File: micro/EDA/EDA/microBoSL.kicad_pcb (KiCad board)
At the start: 4 copper layers, 40 x 13 mm, 37 parts, among them J1 Conn_01x04, J2 Conn_02x03_Odd_Even, J3 Conn_01x04, J4 Conn_01x04, J5 Conn_01x02, J6 Conn_01x10, J7 Conn_01x02, J8 USB_B_Micro, Q1 DMG2302UK, SW1 PTS636 SM43J SMTR LFS, U1 MAX40200ANS, U2 MAX40200ANS, U3 MCP1700-3302E_SOT23, U4 ATmega328-MMH, U5 MCP7940N-xSN, U6 74HC126PW-Q100, U7 FT232RQ, Y1 8MHz, Y2 32.768 kHz

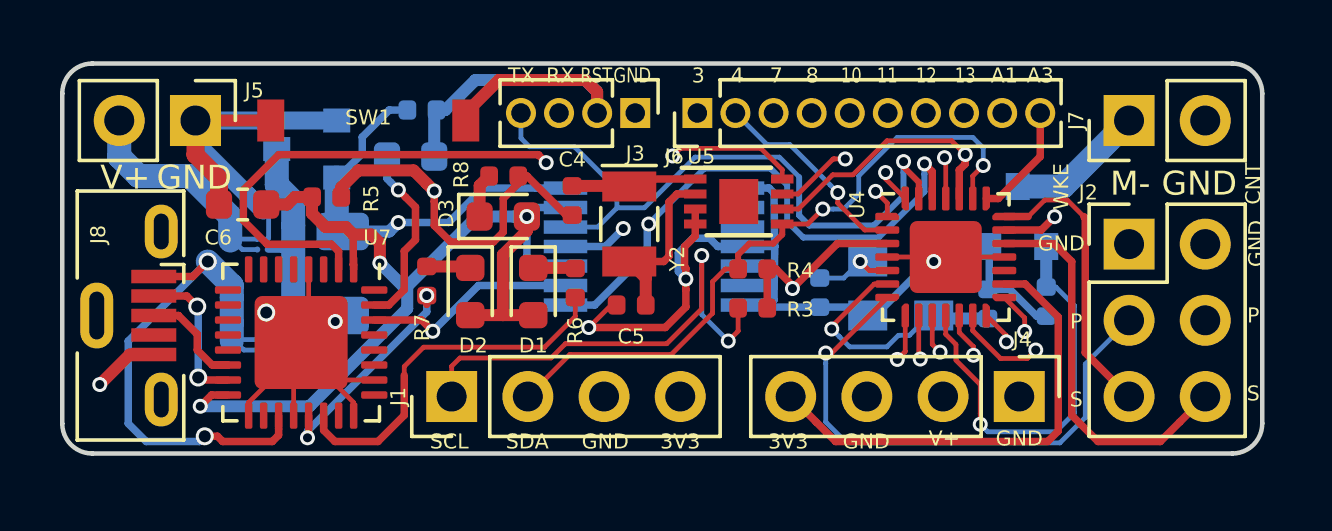
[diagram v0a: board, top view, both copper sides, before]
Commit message: microbosl layout finished TODO: optimise/silkscreen
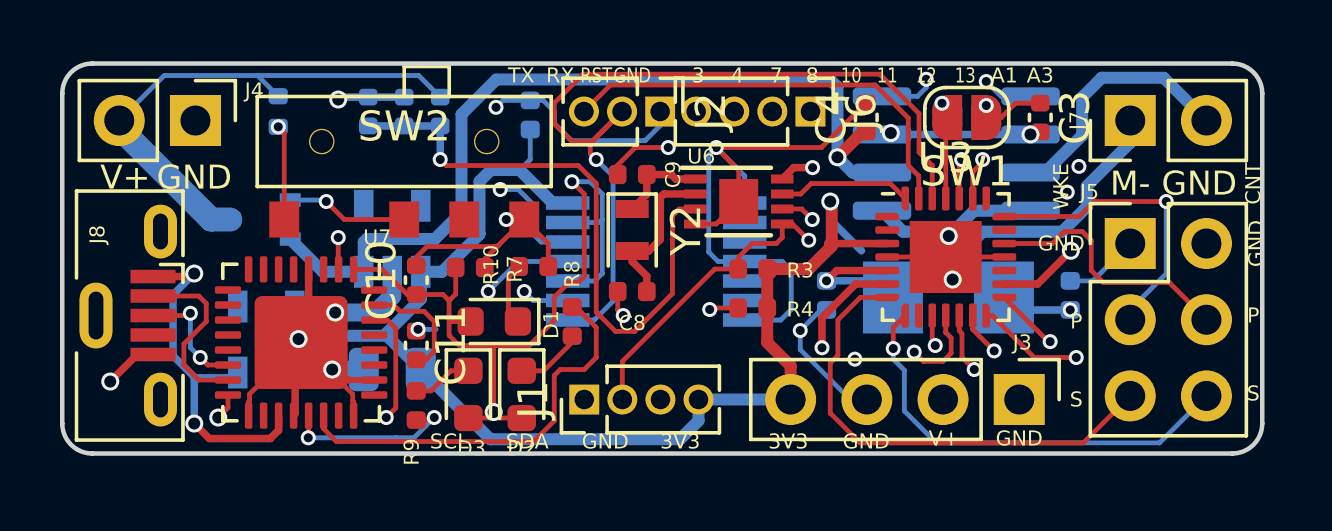
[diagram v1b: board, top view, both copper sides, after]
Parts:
- removed the C6 at (106.0, 106.7)
- removed the D3 at (114.7, 107.1)
- removed the J3 at (119.1, 103.7)
- removed the R2 at (132.8, 109.9)
- added C10: 100 nF, Capacitor_SMD:C_0402_1005Metric, F.Cu at (111.8, 109.2)
- added C11: 100 nF, Capacitor_SMD:C_0402_1005Metric, F.Cu at (111.8, 111.4)
- added C3: 100 nF, Capacitor_SMD:C_0402_1005Metric, F.Cu at (132.6, 103.8)
- added C4: 100 nF, Capacitor_SMD:C_0402_1005Metric, F.Cu at (126.8, 103.8)
- added D2: LED, LED_SMD:LED_0603_1608Metric, F.Cu at (115.3, 113.0)
- added J2: Conn_01x03, Connector_PinHeader_1.27mm:PinHeader_1x03_P1.27mm_Vertical, F.Cu at (119.9, 103.6)
- added R1: 10 kΩ, Resistor_SMD:R_0402_1005Metric, B.Cu at (107.2, 103.6)
- added R6: 4.7 MΩ, Capacitor_SMD:C_0402_1005Metric, B.Cu at (110.2, 103.6)
- added R9: 3.3 kΩ, Resistor_SMD:R_0402_1005Metric, F.Cu at (111.8, 113.4)
- added SW2: AYZ0103AGRLC, SIMFootprints:AYZ0103AGRLC, F.Cu at (111.4, 104.6)
- C1: value 1 μF -> 2.2 μF; footprint Capacitor_SMD:C_1206_3216Metric -> Capacitor_SMD:C_0805_2012Metric
- C5: renamed from C3; value 22 pF -> 15 pF
- C6: renamed from C2; value 22 pF -> 15 pF
- C7: footprint Capacitor_SMD:C_0603_1608Metric -> Capacitor_SMD:C_0402_1005Metric
- C8: renamed from C5; value 12 pF -> 15 pF
- C9: renamed from C4; value 12 pF -> 15 pF
- J1: footprint Connector_PinHeader_2.54mm:PinHeader_1x04_P2.54mm_Vertical -> Connector_PinHeader_1.27mm:PinHeader_1x04_P1.27mm_Vertical
- J4: renamed from J5; value Conn_01x02 -> BATTERY CONN
- J6: value Conn_01x10 -> Conn_01x04; footprint Connector_PinHeader_1.27mm:PinHeader_1x10_P1.27mm_Vertical -> Connector_PinHeader_1.27mm:PinHeader_1x04_P1.27mm_Vertical
- J7: value Conn_01x02 -> MOTOR_OUT
- Q1: value DMG2302UK -> DMP2165UW; footprint Package_TO_SOT_SMD:SOT-23 -> Package_TO_SOT_SMD:SOT-323_SC-70
- R5: value 10 kΩ -> 4.7 MΩ; footprint Resistor_SMD:R_0402_1005Metric -> Capacitor_SMD:C_0402_1005Metric; moved to B.Cu
- R7: value 3.3 kΩ -> 10 kΩ
- SW1: value PTS636 SM43J SMTR LFS -> RST_JMPR; footprint SIMFootprints:PTS636 SM43J SMTR LFS -> Jumper:SolderJumper-2_P1.3mm_Open_RoundedPad1.0x1.5mm
- U1, U2: value MAX40200ANS -> TPS709A33DBVT; footprint Package_BGA:WLP-4_0.73x0.73mm_Layout2x2_P0.35mm_Ball0.22mm_Pad0.2mm_NSMD -> Package_TO_SOT_SMD:SOT-23-5
- U3: value MCP1700-3302E_SOT23 -> ATmega328P-MMH; footprint Package_TO_SOT_SMD:SOT-23 -> Package_DFN_QFN:QFN-28-1EP_4x4mm_P0.45mm_EP2.4x2.4mm; moved to F.Cu
- U4: value ATmega328-MMH -> ZXBM5210-S; footprint Package_DFN_QFN:QFN-28-1EP_4x4mm_P0.45mm_EP2.4x2.4mm -> Package_SO:SOIC-8_3.9x4.9mm_P1.27mm; moved to B.Cu
- Y1: footprint Crystal:Crystal_SMD_EuroQuartz_MT-4Pin_3.2x2.5mm -> Crystal:Crystal_SMD_5032-2Pin_5.0x3.2mm
- Y2: footprint Crystal:Crystal_SMD_EuroQuartz_EQ161-2Pin_3.2x1.5mm -> Crystal:Crystal_SMD_2012-2Pin_2.0x1.2mm
- moved Q1 25.3 mm to (106.6, 107.2), turned to 180 degrees
- moved U3 21.6 mm to (129.4, 108.5), turned to 0 degrees
- moved SW1 20.0 mm to (130.2, 103.8)
- moved R5 4.74 mm to (112.6, 103.6), turned to 270 degrees
- moved J1 4.42 mm to (117.4, 113.2)
- moved U2 4.33 mm to (111.0, 107.8), turned to 90 degrees
- moved J6 3.77 mm to (124.9, 103.6), turned to 270 degrees
- moved R2 3.61 mm to (115.6, 103.7), turned to 90 degrees
- moved C1 3.60 mm to (111.0, 112.2), turned to 180 degrees
- moved U4 3.47 mm to (129.8, 105.0)
- moved D3 3.43 mm to (113.5, 113.0)
- moved R10 3.18 mm to (115.7, 108.8)
- moved C6 2.76 mm to (133.6, 109.7)
- moved C9 2.18 mm to (119.0, 105.7), turned to 0 degrees
- moved D1 1.64 mm to (114.4, 110.6), turned to 180 degrees
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- renumbered D2 to D3, J4 to J3, J2 to J5, R8 to R10, R1 to R2, R4 to R3, R3 to R4, R6 to R8, U6 to U5, U5 to U6
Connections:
- C5 pad 2: Net-(C3-Pad2) -> Net-(C5-Pad2)
- C6 pad 2: Net-(C2-Pad2) -> Net-(C6-Pad2)
- C7 pad 1: TLL_RST -> Net-(C7-Pad1)
- C7 pad 2: Net-(C7-Pad2) -> GND
- D3 pad 1: Net-(D2-Pad1) -> Net-(D3-Pad1)
- J3 pad 2: VPP -> VBAT
- J5 pad 3: Hall_WKE_P -> Hall_WKE_S
- J5 pad 4: Hall_CNT_P -> Hall_CNT_S
- J5 pad 5: Hall_WKE_S -> Hall_WKE_P
- J5 pad 6: Hall_CNT_S -> Hall_CNT_P
- J6 pad 1: D3 -> SCLK
- J6 pad 2: D4 -> MISO
- J6 pad 3: D7 -> MOSI
- J6 pad 4: D8 -> SS
- J7 pad 2: GND -> Net-(J7-Pad2)
- Q1 pad 1: MOSFET -> Net-(Q1-Pad1)
- Q1 pad 2: GND -> VBAT
- Q1 pad 3: Net-(J7-Pad1) -> VPP
- R10 pad 1: Net-(D3-Pad1) -> Net-(D1-Pad1)
- R5 pad 1: TTL_3.3V -> VPP
- R5 pad 2: GND -> Net-(C7-Pad1)
- R7 pad 1: Net-(D2-Pad1) -> TTL_3.3V
- R7 pad 2: Net-(R7-Pad2) -> GND
- R8 pad 1: Net-(D1-Pad1) -> Net-(D2-Pad1)
- U3 pad 1: GND -> D3
- U3 pad 2: V_3.3 -> D4
- U3 pad 3: Net-(U1-PadA2) -> V_3.3
- U4 pad 1: D3 -> Net-(J7-Pad1)
- U4 pad 2: D4 -> VBAT
- U4 pad 4: GND -> MFWD
- U4 pad 5: Net-(C3-Pad2) -> MREV
- U4 pad 6: Net-(C2-Pad2) -> V_3.3
- U4 pad 7: Hall_WKE_P -> Net-(J7-Pad2)
- U4 pad 8: Hall_CNT_P -> GND
- U6 pad 3: GND -> Net-(C7-Pad1)
- U6 pad 9: (no net) -> GND
- U7 pad 21: Net-(R7-Pad2) -> Net-(R9-Pad2)
- U7 pad 31: Net-(C7-Pad2) -> Net-(C11-Pad2)
- Y1 pad 1: Net-(C2-Pad2) -> Net-(C6-Pad2)
- Y1 pad 2: GND -> Net-(C5-Pad2)
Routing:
- net VBAT: track 0.00 -> 43.3 mm, vias 0 -> 1
- net VPP: track 43.6 -> 17.8 mm
- net MISO: track 0.00 -> 21.6 mm, vias 0 -> 2
- net SS: track 0.00 -> 21.2 mm, vias 0 -> 1
- net Net-(C7-Pad1): track 0.00 -> 20.1 mm, vias 0 -> 1
- net SCLK: track 0.00 -> 19.1 mm, vias 0 -> 2
- net MOSI: track 0.00 -> 16.4 mm, vias 0 -> 2
- net SCL: track 35.5 -> 19.3 mm
- net D11: track 15.0 -> 0.00 mm, vias 1 -> 0
- net Net-(C6-Pad2): track 0.00 -> 14.8 mm, vias 0 -> 2
- net MFWD: track 0.00 -> 13.9 mm, vias 0 -> 2
- net MOSFET: track 13.7 -> 0.00 mm, vias 1 -> 0
- net D10: track 13.1 -> 0.00 mm, vias 1 -> 0
- net MREV: track 0.00 -> 12.5 mm, vias 0 -> 2
- net D7: track 12.3 -> 0.00 mm, vias 1 -> 0
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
